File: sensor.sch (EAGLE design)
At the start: 147 parts, among them CN1 FH52E-60S-0.5SH, CN2 TC2030, U1 GMAX0505-DV, U10 EMC1812T, U2 STM32L031G6, U3 MP2148, U4 MAX25300B, U5 MAX25300B, U6 MAX25300B, U7 MAX25300B, U8 LM2662, U9 MAX1735

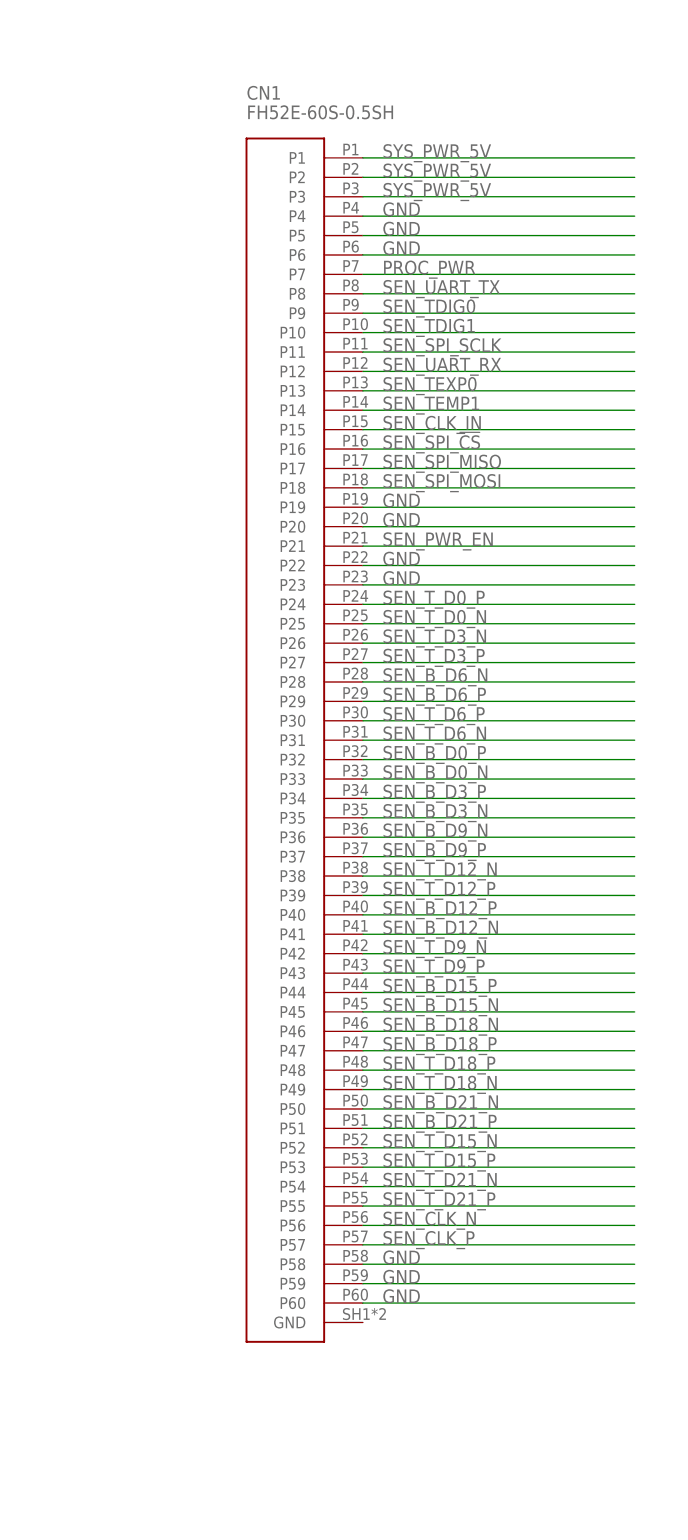
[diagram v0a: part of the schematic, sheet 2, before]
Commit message: Mech design and layout
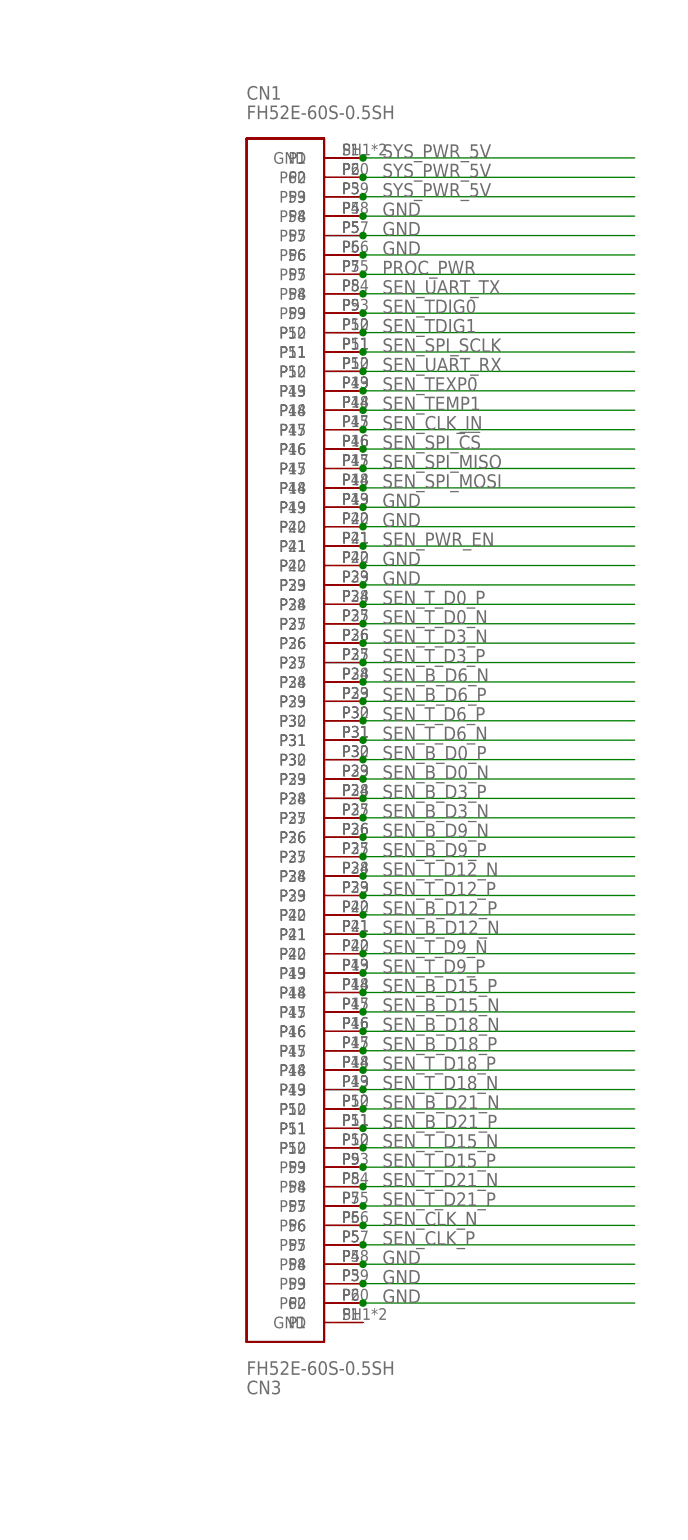
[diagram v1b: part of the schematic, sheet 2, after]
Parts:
- added CN3: FH52E-60S-0.5SH, CONNECTORs:FH52E-60S-0.5SH
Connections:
- new net N$5: CN1.GND, CN3.P1
- net GND: now also CN3.P2, CN3.P3, CN3.P39, CN3.P4, CN3.P40, CN3.P42, CN3.P43, CN3.P56, CN3.P57, CN3.P58
- net PROC_PWR: now also CN3.P55
- net SEN_B_D0_N: now also CN3.P29
- net SEN_B_D0_P: now also CN3.P30
- net SEN_B_D12_N: now also CN3.P21
- net SEN_B_D12_P: now also CN3.P22
- net SEN_B_D15_N: now also CN3.P17
- net SEN_B_D15_P: now also CN3.P18
- net SEN_B_D18_N: now also CN3.P16
- net SEN_B_D18_P: now also CN3.P15
- net SEN_B_D21_N: now also CN3.P12
- net SEN_B_D21_P: now also CN3.P11
- net SEN_B_D3_N: now also CN3.P27
- net SEN_B_D3_P: now also CN3.P28
- net SEN_B_D6_N: now also CN3.P34
- net SEN_B_D6_P: now also CN3.P33
- net SEN_B_D9_N: now also CN3.P26
- net SEN_B_D9_P: now also CN3.P25
- net SEN_CLK_IN: now also CN3.P47
- net SEN_CLK_N: now also CN3.P6
- net SEN_CLK_P: now also CN3.P5
- net SEN_PWR_EN: now also CN3.P41
- net SEN_SPI_!CS: now also CN3.P46
- net SEN_SPI_MISO: now also CN3.P45
- net SEN_SPI_MOSI: now also CN3.P44
- net SEN_SPI_SCLK: now also CN3.P51
- net SEN_TDIG0: now also CN3.P53
- net SEN_TDIG1: now also CN3.P52
- net SEN_TEMP1: now also CN3.P48
- net SEN_TEXP0: now also CN3.P49
- net SEN_T_D0_N: now also CN3.P37
- net SEN_T_D0_P: now also CN3.P38
- net SEN_T_D12_N: now also CN3.P24
- net SEN_T_D12_P: now also CN3.P23
- net SEN_T_D15_N: now also CN3.P10
- net SEN_T_D15_P: now also CN3.P9
- net SEN_T_D18_N: now also CN3.P13
- net SEN_T_D18_P: now also CN3.P14
- net SEN_T_D21_N: now also CN3.P8
- net SEN_T_D21_P: now also CN3.P7
- net SEN_T_D3_N: now also CN3.P36
- net SEN_T_D3_P: now also CN3.P35
- net SEN_T_D6_N: now also CN3.P31
- net SEN_T_D6_P: now also CN3.P32
- net SEN_T_D9_N: now also CN3.P20
- net SEN_T_D9_P: now also CN3.P19
- net SEN_UART_RX: now also CN3.P50
- net SEN_UART_TX: now also CN3.P54
- net SYS_PWR_5V: now also CN3.GND, CN3.P59, CN3.P60

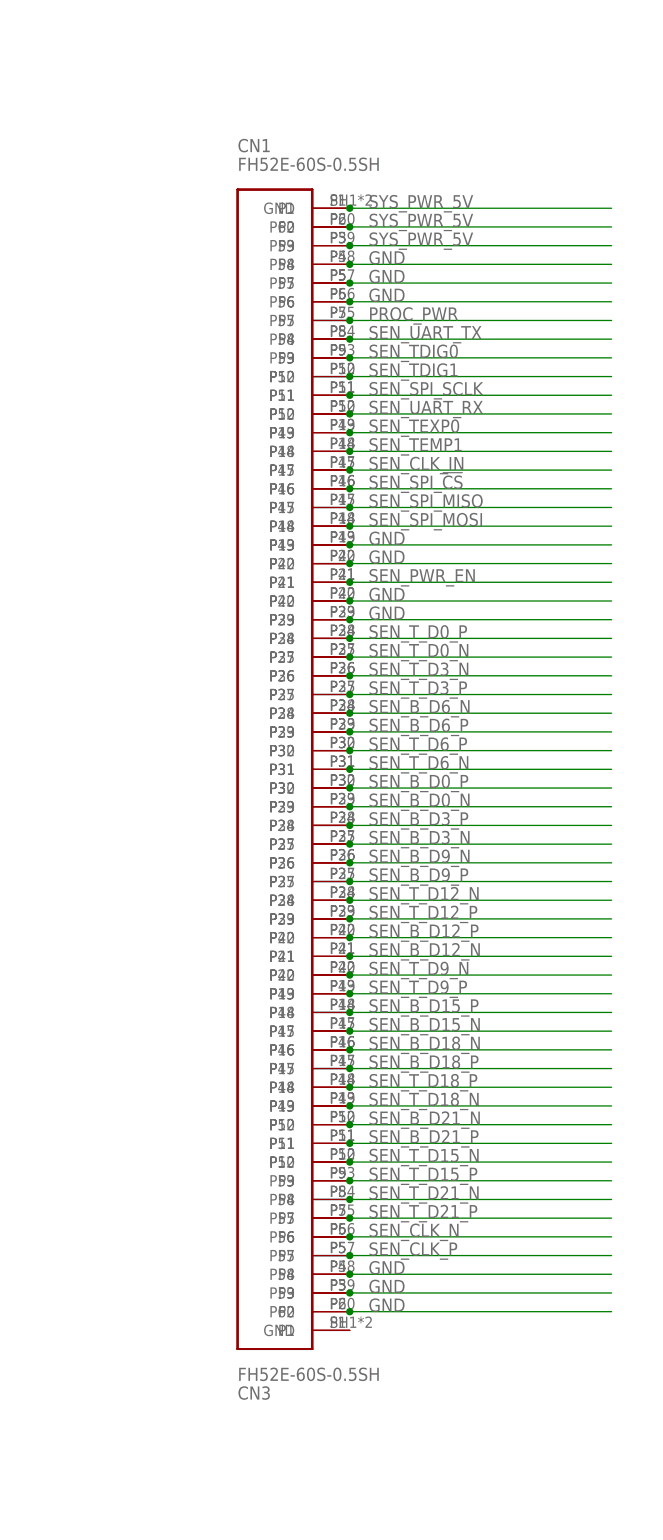
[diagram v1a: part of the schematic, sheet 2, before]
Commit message: Moved to FT600 due to IO constraints
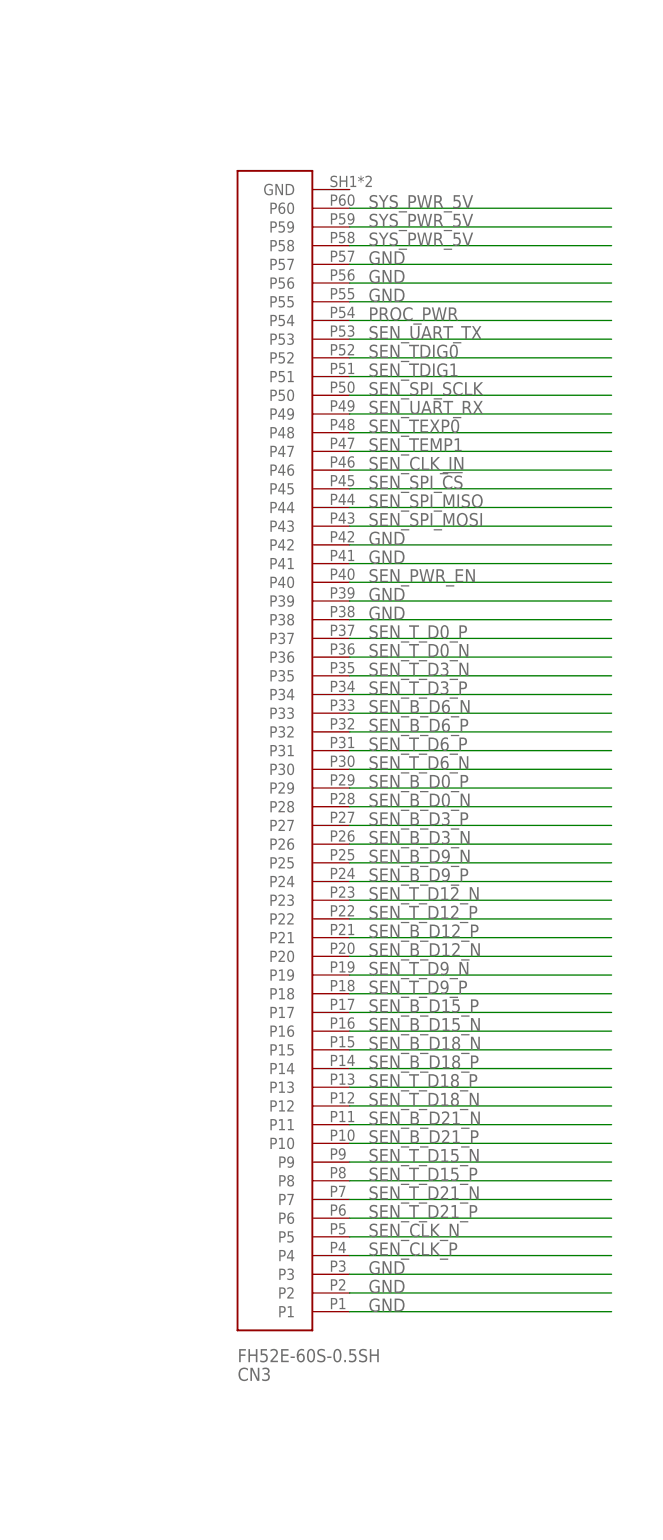
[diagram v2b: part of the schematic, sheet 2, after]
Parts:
- removed CN1: FH52E-60S-0.5SH, CONNECTORs:FH52E-60S-0.5SH
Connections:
- removed net N$5: CN1.GND, CN3.P1
- net GND: now also CN3.P1, CN3.P38, CN3.P41, CN3.P55; no longer CN1.P19, CN1.P20, CN1.P22, CN1.P23, CN1.P4, CN1.P5, CN1.P58, CN1.P59, CN1.P6, CN1.P60, CN3.P4, CN3.P40, CN3.P43, CN3.P58
- net PROC_PWR: now also CN3.P54; no longer CN1.P7, CN3.P55
- net SEN_B_D0_N: now also CN3.P28; no longer CN1.P33, CN3.P29
- net SEN_B_D0_P: now also CN3.P29; no longer CN1.P32, CN3.P30
- net SEN_B_D12_N: now also CN3.P20; no longer CN1.P41, CN3.P21
- net SEN_B_D12_P: now also CN3.P21; no longer CN1.P40, CN3.P22
- net SEN_B_D15_N: now also CN3.P16; no longer CN1.P45, CN3.P17
- net SEN_B_D15_P: now also CN3.P17; no longer CN1.P44, CN3.P18
- net SEN_B_D18_N: now also CN3.P15; no longer CN1.P46, CN3.P16
- net SEN_B_D18_P: now also CN3.P14; no longer CN1.P47, CN3.P15
- net SEN_B_D21_N: now also CN3.P11; no longer CN1.P50, CN3.P12
- net SEN_B_D21_P: now also CN3.P10; no longer CN1.P51, CN3.P11
- net SEN_B_D3_N: now also CN3.P26; no longer CN1.P35, CN3.P27
- net SEN_B_D3_P: now also CN3.P27; no longer CN1.P34, CN3.P28
- net SEN_B_D6_N: now also CN3.P33; no longer CN1.P28, CN3.P34
- net SEN_B_D6_P: now also CN3.P32; no longer CN1.P29, CN3.P33
- net SEN_B_D9_N: now also CN3.P25; no longer CN1.P36, CN3.P26
- net SEN_B_D9_P: now also CN3.P24; no longer CN1.P37, CN3.P25
- net SEN_CLK_IN: now also CN3.P46; no longer CN1.P15, CN3.P47
- net SEN_CLK_N: now also CN3.P5; no longer CN1.P56, CN3.P6
- net SEN_CLK_P: now also CN3.P4; no longer CN1.P57, CN3.P5
- net SEN_PWR_EN: now also CN3.P40; no longer CN1.P21, CN3.P41
- net SEN_SPI_!CS: now also CN3.P45; no longer CN1.P16, CN3.P46
- net SEN_SPI_MISO: now also CN3.P44; no longer CN1.P17, CN3.P45
- net SEN_SPI_MOSI: now also CN3.P43; no longer CN1.P18, CN3.P44
- net SEN_SPI_SCLK: now also CN3.P50; no longer CN1.P11, CN3.P51
- net SEN_TDIG0: now also CN3.P52; no longer CN1.P9, CN3.P53
- net SEN_TDIG1: now also CN3.P51; no longer CN1.P10, CN3.P52
- net SEN_TEMP1: now also CN3.P47; no longer CN1.P14, CN3.P48
- net SEN_TEXP0: now also CN3.P48; no longer CN1.P13, CN3.P49
- net SEN_T_D0_N: now also CN3.P36; no longer CN1.P25, CN3.P37
- net SEN_T_D0_P: now also CN3.P37; no longer CN1.P24, CN3.P38
- net SEN_T_D12_N: now also CN3.P23; no longer CN1.P38, CN3.P24
- net SEN_T_D12_P: now also CN3.P22; no longer CN1.P39, CN3.P23
- net SEN_T_D15_N: now also CN3.P9; no longer CN1.P52, CN3.P10
- net SEN_T_D15_P: now also CN3.P8; no longer CN1.P53, CN3.P9
- net SEN_T_D18_N: now also CN3.P12; no longer CN1.P49, CN3.P13
- net SEN_T_D18_P: now also CN3.P13; no longer CN1.P48, CN3.P14
- net SEN_T_D21_N: now also CN3.P7; no longer CN1.P54, CN3.P8
- net SEN_T_D21_P: now also CN3.P6; no longer CN1.P55, CN3.P7
- net SEN_T_D3_N: now also CN3.P35; no longer CN1.P26, CN3.P36
- net SEN_T_D3_P: now also CN3.P34; no longer CN1.P27, CN3.P35
- net SEN_T_D6_N: now also CN3.P30; no longer CN1.P31, CN3.P31
- net SEN_T_D6_P: now also CN3.P31; no longer CN1.P30, CN3.P32
- net SEN_T_D9_N: now also CN3.P19; no longer CN1.P42, CN3.P20
- net SEN_T_D9_P: now also CN3.P18; no longer CN1.P43, CN3.P19
- net SEN_UART_RX: now also CN3.P49; no longer CN1.P12, CN3.P50
- net SEN_UART_TX: now also CN3.P53; no longer CN1.P8, CN3.P54
- net SYS_PWR_5V: now also CN3.P58; no longer CN1.P1, CN1.P2, CN1.P3, CN3.GND
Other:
- moved on the sheet: CN3
